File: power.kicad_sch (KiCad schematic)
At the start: 12 parts, among them U3 TPS61170DRVR

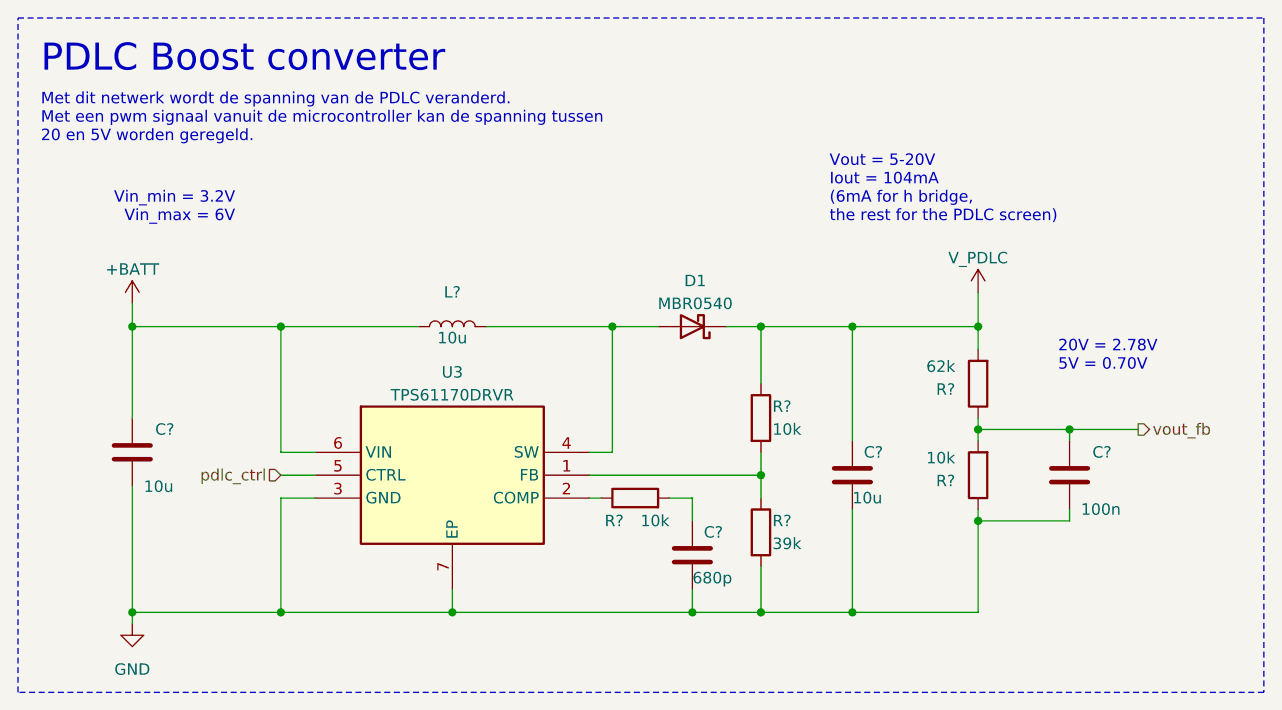
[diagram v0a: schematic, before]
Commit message: footprint assignments gedaan + verbeteringen
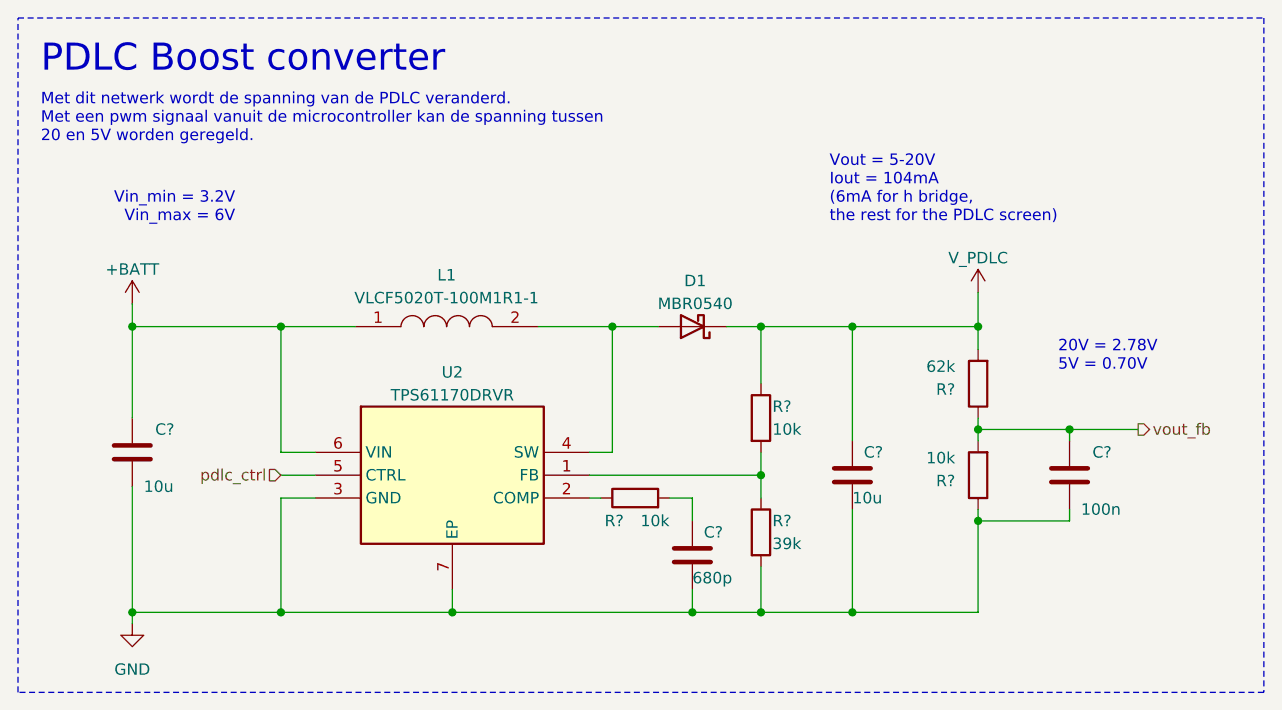
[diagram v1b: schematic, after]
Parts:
- removed L?: 10u, symbol Device:L
- added L1: VLCF5020T-100M1R1-1, VLCF5020, symbol SamacSys_Parts:VLCF5020T-100M1R1-1
- C? (x4): footprint (none) -> Capacitor_SMD:C_0805_2012Metric_Pad1.18x1.45mm_HandSolder
- renumbered U3 to U2
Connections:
- net +BATT: now also L1.1
- net at D1.2 (A), U2.4 (SW): now also L1.2
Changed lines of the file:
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@@
   (junction (at 206.375 107.315) (diameter 0) (color 0 0 0 0)
   )
+  (junction (at 155.575 95.885) (diameter 0) (color 0 0 0 0)
+  )
   (junction (at 196.215 117.475) (diameter 0) (color 0 0 0 0)
   )
@@
   )
   (junction (at 196.215 95.885) (diameter 0) (color 0 0 0 0)
-  )
-  (junction (at 155.575 95.885) (diameter 0) (color 0 0 0 0)
   )
   (junction (at 172.085 95.885) (diameter 0) (color 0 0 0 0)
@@
     (stroke (width 0) (type dash))
   )
-  (wire (pts (xy 141.605 95.885) (xy 155.575 95.885))
-    (stroke (width 0) (type default))
-  )
-  (wire (pts (xy 118.745 95.885) (xy 133.985 95.885))
-    (stroke (width 0) (type default))
-  )
   (wire (pts (xy 172.085 112.395) (xy 172.085 114.935))
     (stroke (width 0) (type default))
@@
     (stroke (width 0) (type dash))
   )
+  (wire (pts (xy 118.745 95.885) (xy 127 95.885))
+    (stroke (width 0) (type default))
+  )
   (wire (pts (xy 155.575 95.885) (xy 155.575 109.855))
     (stroke (width 0) (type default))
@@
   )
   (wire (pts (xy 164.465 127.635) (xy 172.085 127.635))
+    (stroke (width 0) (type default))
+  )
+  (wire (pts (xy 147.32 95.885) (xy 155.575 95.885))
     (stroke (width 0) (type default))
   )
@@
         )
         (path "/5dc439a9-720d-4bdc-b61f-78a76fde4df5/2d26b15a-54d8-4f7d-a410-dc25ffe321a1"
-          (reference "R8") (unit 1)
+          (reference "R12") (unit 1)
         )
       )
@@
       (effects (font (size 1.27 1.27)) (justify left))
     )
-    (property "Footprint" "" (at 183.2102 116.205 0)
+    (property "Footprint" "Capacitor_SMD:C_0805_2012Metric_Pad1.18x1.45mm_HandSolder" (at 183.2102 116.205 0)
       (effects (font (size 1.27 1.27)) hide)
     )
@@
         )
         (path "/5dc439a9-720d-4bdc-b61f-78a76fde4df5/2d26b15a-54d8-4f7d-a410-dc25ffe321a1"
-          (reference "C11") (unit 1)
+          (reference "C7") (unit 1)
         )
       )
@@
   (symbol (lib_id "CustomSymbols:V_PDLC") (at 196.215 92.075 0) (unit 1)
     (in_bom yes) (on_board yes) (dnp no) (fields_autoplaced)
-    (property "Reference" "#PWR036" (at 196.215 95.885 0)
+    (property "Reference" "#PWR027" (at 196.215 95.885 0)
       (effects (font (size 1.27 1.27)) hide)
     )
@@
       (project "RookBril"
         (path "/5dc439a9-720d-4bdc-b61f-78a76fde4df5/2d26b15a-54d8-4f7d-a410-dc25ffe321a1"
-          (reference "#PWR036") (unit 1)
-        )
-      )
-    )
-  )
-  (symbol (lib_id "Device:L") (at 137.795 95.885 270) (mirror x) (unit 1)
-    (in_bom yes) (on_board yes) (dnp no)
-    (property "Reference" "L?" (at 137.795 92.075 90)
-      (effects (font (size 1.27 1.27)))
-    )
-    (property "Value" "10u" (at 137.795 97.155 90)
-      (effects (font (size 1.27 1.27)))
-    )
-    (property "Footprint" "" (at 137.795 95.885 0)
-      (effects (font (size 1.27 1.27)) hide)
-    )
-    (property "Datasheet" "~" (at 137.795 95.885 0)
-      (effects (font (size 1.27 1.27)) hide)
-    )
-    (pin "1")
-    (pin "2")
-    (instances
-      (project "RookBril"
-        (path "/5dc439a9-720d-4bdc-b61f-78a76fde4df5"
-          (reference "L?") (unit 1)
-        )
-        (path "/5dc439a9-720d-4bdc-b61f-78a76fde4df5/2d26b15a-54d8-4f7d-a410-dc25ffe321a1"
-          (reference "L1") (unit 1)
+          (reference "#PWR027") (unit 1)
         )
       )
@@
   (symbol (lib_id "power:GND") (at 102.235 128.905 0) (unit 1)
     (in_bom yes) (on_board yes) (dnp no) (fields_autoplaced)
-    (property "Reference" "#PWR038" (at 102.235 135.255 0)
+    (property "Reference" "#PWR029" (at 102.235 135.255 0)
       (effects (font (size 1.27 1.27)) hide)
     )
@@
       (project "RookBril"
         (path "/5dc439a9-720d-4bdc-b61f-78a76fde4df5/2d26b15a-54d8-4f7d-a410-dc25ffe321a1"
-          (reference "#PWR038") (unit 1)
+          (reference "#PWR029") (unit 1)
         )
       )
@@
         )
         (path "/5dc439a9-720d-4bdc-b61f-78a76fde4df5/2d26b15a-54d8-4f7d-a410-dc25ffe321a1"
-          (reference "R4") (unit 1)
+          (reference "R8") (unit 1)
         )
       )
@@
       (effects (font (size 1.27 1.27)) (justify left))
     )
-    (property "Footprint" "" (at 103.2002 113.665 0)
+    (property "Footprint" "Capacitor_SMD:C_0805_2012Metric_Pad1.18x1.45mm_HandSolder" (at 103.2002 113.665 0)
       (effects (font (size 1.27 1.27)) hide)
     )
@@
         )
         (path "/5dc439a9-720d-4bdc-b61f-78a76fde4df5/2d26b15a-54d8-4f7d-a410-dc25ffe321a1"
-          (reference "C10") (unit 1)
+          (reference "C6") (unit 1)
         )
       )
@@
         )
         (path "/5dc439a9-720d-4bdc-b61f-78a76fde4df5/2d26b15a-54d8-4f7d-a410-dc25ffe321a1"
-          (reference "R7") (unit 1)
+          (reference "R11") (unit 1)
         )
       )
@@
   (symbol (lib_id "power:+BATT") (at 102.235 93.345 0) (unit 1)
     (in_bom yes) (on_board yes) (dnp no) (fields_autoplaced)
-    (property "Reference" "#PWR037" (at 102.235 97.155 0)
+    (property "Reference" "#PWR028" (at 102.235 97.155 0)
       (effects (font (size 1.27 1.27)) hide)
     )
@@
       (project "RookBril"
         (path "/5dc439a9-720d-4bdc-b61f-78a76fde4df5/2d26b15a-54d8-4f7d-a410-dc25ffe321a1"
-          (reference "#PWR037") (unit 1)
+          (reference "#PWR028") (unit 1)
         )
       )
@@
         )
         (path "/5dc439a9-720d-4bdc-b61f-78a76fde4df5/2d26b15a-54d8-4f7d-a410-dc25ffe321a1"
-          (reference "R6") (unit 1)
+          (reference "R10") (unit 1)
         )
       )
@@
       (effects (font (size 1.27 1.27)) (justify left))
     )
-    (property "Footprint" "" (at 207.3402 116.205 0)
+    (property "Footprint" "Capacitor_SMD:C_0805_2012Metric_Pad1.18x1.45mm_HandSolder" (at 207.3402 116.205 0)
       (effects (font (size 1.27 1.27)) hide)
     )
@@
         )
         (path "/5dc439a9-720d-4bdc-b61f-78a76fde4df5/2d26b15a-54d8-4f7d-a410-dc25ffe321a1"
-          (reference "C12") (unit 1)
+          (reference "C8") (unit 1)
         )
       )
@@
         )
         (path "/5dc439a9-720d-4bdc-b61f-78a76fde4df5/2d26b15a-54d8-4f7d-a410-dc25ffe321a1"
-          (reference "R5") (unit 1)
+          (reference "R9") (unit 1)
         )
       )
@@
       (effects (font (size 1.27 1.27)) (justify left))
     )
-    (property "Footprint" "" (at 165.4302 125.095 0)
+    (property "Footprint" "Capacitor_SMD:C_0805_2012Metric_Pad1.18x1.45mm_HandSolder" (at 165.4302 125.095 0)
       (effects (font (size 1.27 1.27)) hide)
     )
@@
         )
         (path "/5dc439a9-720d-4bdc-b61f-78a76fde4df5/2d26b15a-54d8-4f7d-a410-dc25ffe321a1"
-          (reference "C13") (unit 1)
+          (reference "C9") (unit 1)
         )
       )
@@
     )
   )
+  (symbol (lib_id "SamacSys_Parts:VLCF5020T-100M1R1-1") (at 127 95.885 0) (unit 1)
+    (in_bom yes) (on_board yes) (dnp no) (fields_autoplaced)
+    (property "Reference" "L1" (at 137.16 90.17 0)
+      (effects (font (size 1.27 1.27)))
+    )
+    (property "Value" "VLCF5020T-100M1R1-1" (at 137.16 92.71 0)
+      (effects (font (size 1.27 1.27)))
+    )
+    (property "Footprint" "VLCF5020" (at 143.51 94.615 0)
+      (effects (font (size 1.27 1.27)) (justify left) hide)
+    )
+    (property "Datasheet" "https://product.tdk.com/system/files/dam/doc/product/inductor/inductor/smd/catalog/inductor_commercial_power_vlcf5020-1_en.pdf" (at 143.51 97.155 0)
+      (effects (font (size 1.27 1.27)) (justify left) hide)
+    )
+    (property "Description" "TDK VLC5020 Series Shielded Wire-wound SMD Inductor 10 uH +/-20% 1.5A Idc" (at 143.51 99.695 0)
+      (effects (font (size 1.27 1.27)) (justify left) hide)
+    )
+    (property "Height" "" (at 143.51 102.235 0)
+      (effects (font (size 1.27 1.27)) (justify left) hide)
+    )
+    (property "Mouser Part Number" "810-VLCF52T100M1R11" (at 143.51 104.775 0)
+      (effects (font (size 1.27 1.27)) (justify left) hide)
+    )
+    (property "Mouser Price/Stock" "https://www.mouser.co.uk/ProductDetail/TDK/VLCF5020T-100M1R1-1?qs=O2qRfqcg9D93TlFS8ggxKg%3D%3D" (at 143.51 107.315 0)
+      (effects (font (size 1.27 1.27)) (justify left) hide)
+    )
+    (property "Manufacturer_Name" "TDK" (at 143.51 109.855 0)
+      (effects (font (size 1.27 1.27)) (justify left) hide)
+    )
+    (property "Manufacturer_Part_Number" "VLCF5020T-100M1R1-1" (at 143.51 112.395 0)
+      (effects (font (size 1.27 1.27)) (justify left) hide)
+    )
+    (pin "1")
+    (pin "2")
+    (instances
+      (project "RookBril"
+        (path "/5dc439a9-720d-4bdc-b61f-78a76fde4df5/2d26b15a-54d8-4f7d-a410-dc25ffe321a1"
+          (reference "L1") (unit 1)
+        )
+      )
+    )
+  )
   (symbol (lib_id "CustomSymbols:TPS61170DRVR") (at 122.555 107.315 0) (unit 1)
     (in_bom yes) (on_board yes) (dnp no) (fields_autoplaced)
-    (property "Reference" "U3" (at 137.795 100.965 0)
+    (property "Reference" "U2" (at 137.795 100.965 0)
       (effects (font (size 1.27 1.27)))
     )
@@
       (project "RookBril"
         (path "/5dc439a9-720d-4bdc-b61f-78a76fde4df5/2d26b15a-54d8-4f7d-a410-dc25ffe321a1"
-          (reference "U3") (unit 1)
-        )
-      )
+          (reference "U2") (unit 1)
+        )
+      )

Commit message: aantal componenten veranderd.
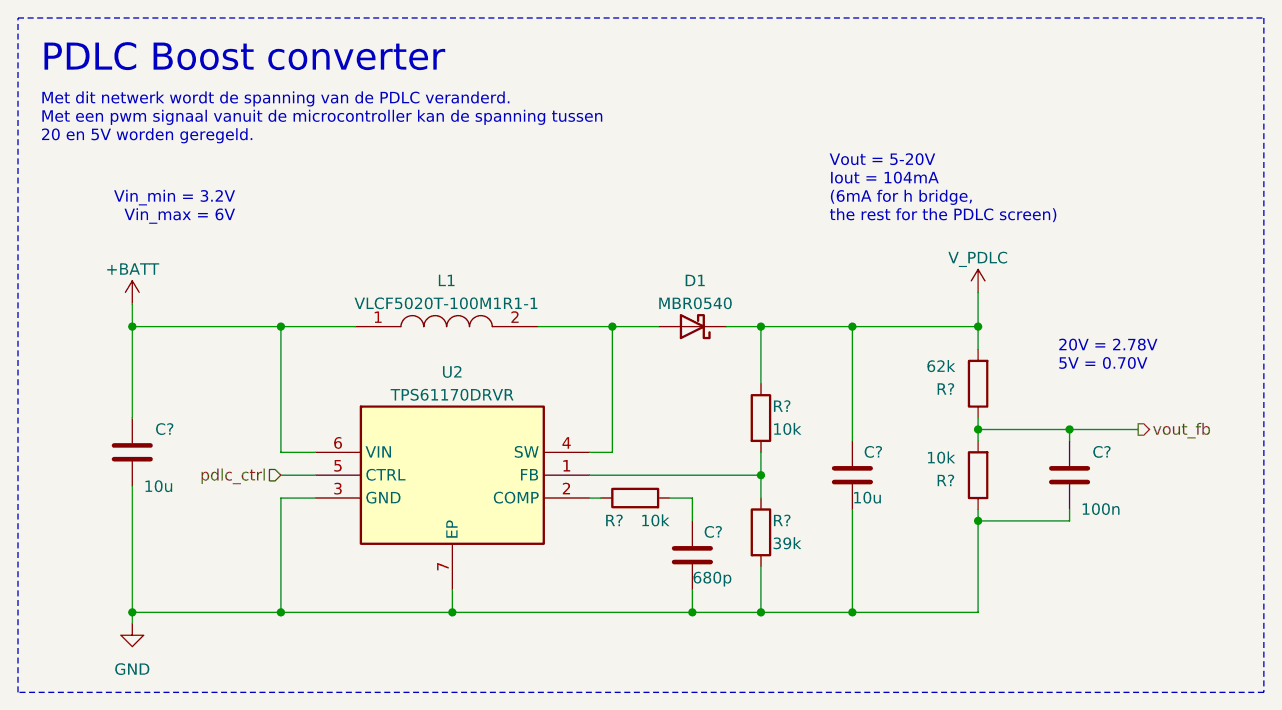
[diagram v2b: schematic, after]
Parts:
- removed L1: VLCF5020T-100M1R1-1, VLCF5020, symbol SamacSys_Parts:VLCF5020T-100M1R1-1
- added L1: VLCF5020T-100M1R1-1, Components:VLCF5020, symbol CustomSymbols:VLCF5020T-100M1R1-1
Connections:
- net +BATT: now also L1.1
- net at D1.2 (A), U2.4 (SW): now also L1.2

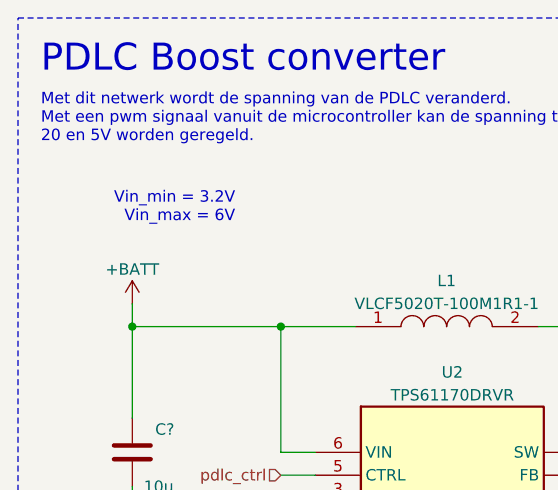
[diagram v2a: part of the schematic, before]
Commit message: nieuwe layout
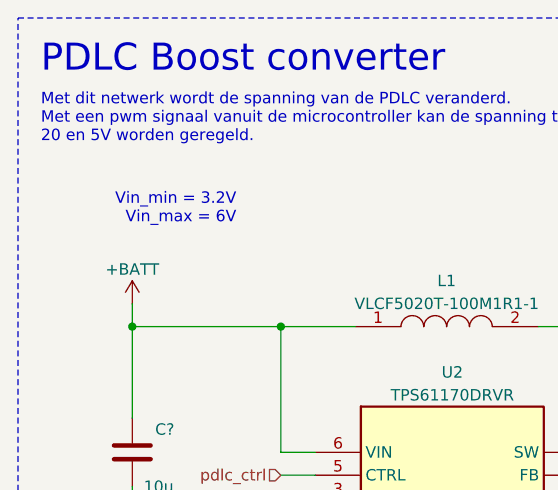
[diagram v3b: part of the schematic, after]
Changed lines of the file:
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@@
     (effects (font (size 1.27 1.27)) (justify left bottom))
   )
-  (text "Vin_min = 3.2V\nVin_max = 6V" (at 113.665 84.455 0)
+  (text "Vin_min = 3.2V\nVin_max = 6V" (at 113.792 84.582 0)
     (effects (font (size 1.27 1.27)) (justify right bottom))
   )
